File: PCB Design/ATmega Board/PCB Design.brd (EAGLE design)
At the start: 96.3 x 64.3 mm, 33 parts

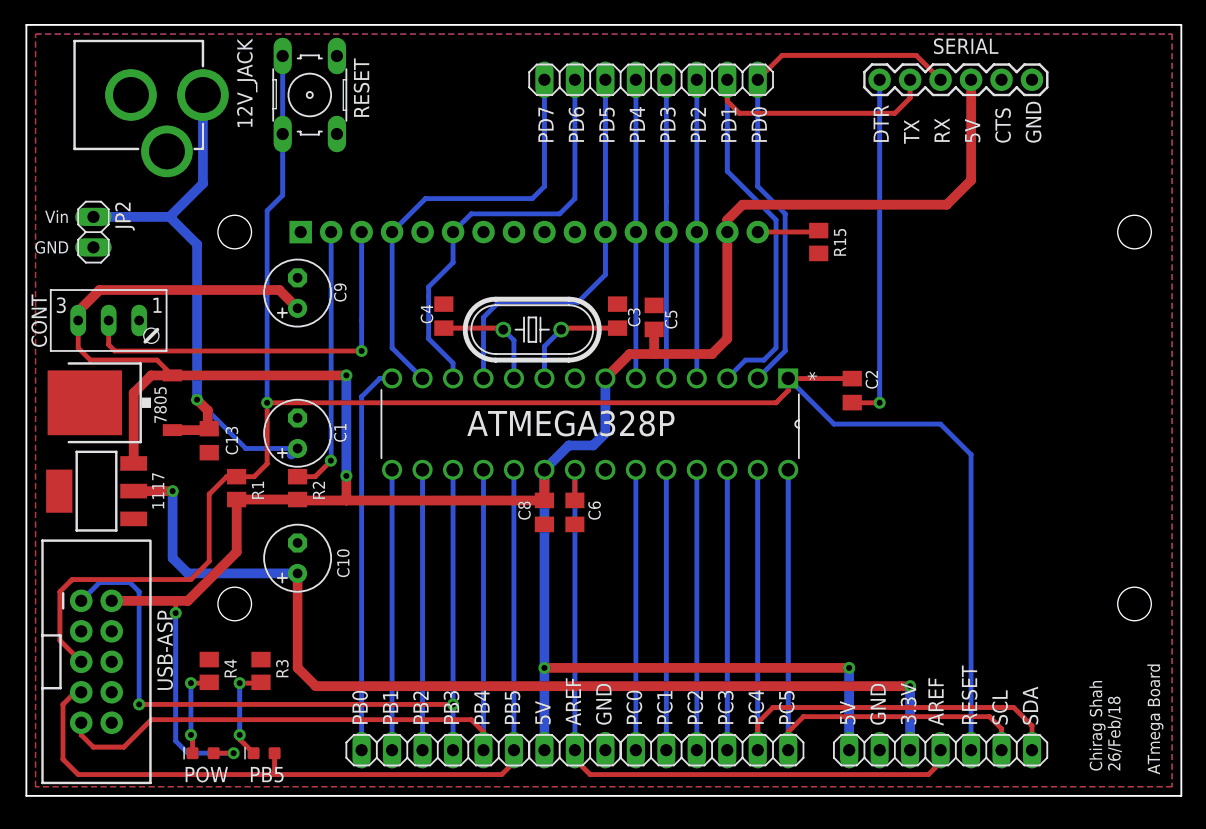
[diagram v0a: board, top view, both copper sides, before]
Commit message: Before renumbering parts
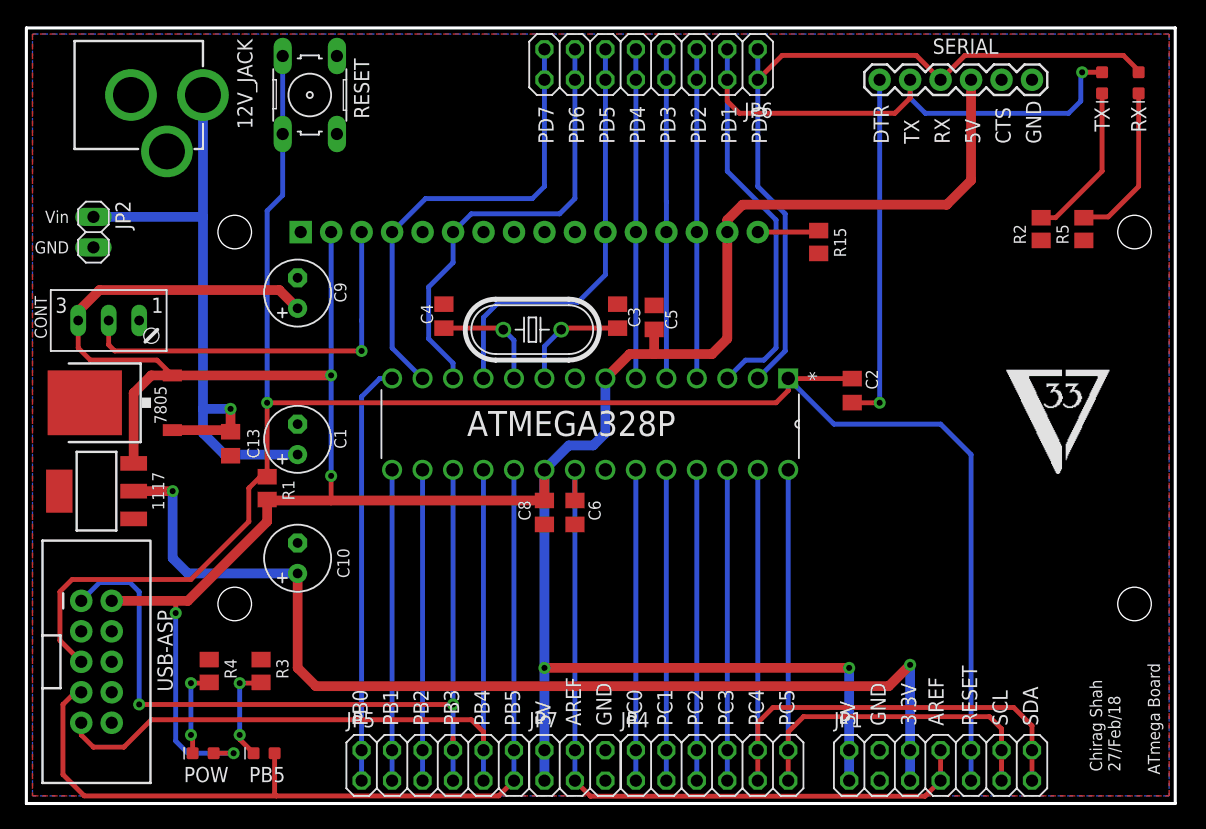
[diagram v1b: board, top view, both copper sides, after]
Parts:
- removed JP3: (no value), pinhead:1X07
- removed PORT_B, PORT_C: (no value), pinhead:1X06
- removed PORT_D: (no value), pinhead:1X08
- added JP4, JP5: (no value), pinhead:2X06
- added JP6: (no value), pinhead:2X08
- added JP7: (no value), pinhead:2X03
- added R5: 330, resistor:M0805
- added RX, TX: BLUE, SparkFun-LED:LED-0603
- JP1: device pinhead:1X03 -> pinhead:2X07
- R2: value 220 -> 330
- moved R2 65.6 mm to (91.9, 53.6)
- moved JP1 30.5 mm to (83.6, 8.89)
- moved R1 2.54 mm to (27.4, 32.0)
- moved C13 1.80 mm to (24.4, 35.7)
- moved C1 0.51 mm to (30.0, 36.1)
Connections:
- new net N$3: R5.2, RX.C
- net +5V: now also JP1.2, JP7.1, JP7.2, LCD.2; no longer JP3.1, R2.1
- net 3.3V: now also JP1.5, JP1.6; no longer JP3.3
- net AREF: now also JP1.7, JP1.8, JP7.3, JP7.4; no longer JP1.2, JP3.4
- net GND: now also JP1.4, JP7.5, JP7.6, R2.1, R5.1; no longer JP3.2
- net N$7: now also TX.C; no longer LCD.2
- net PB0/D8: now also JP5.1, JP5.2; no longer PORT_B.1
- net PB1/D9: now also JP5.3, JP5.4; no longer PORT_B.2
- net PB2/D10: now also JP5.5, JP5.6; no longer PORT_B.3
- net PB3/MOSI/D11: now also JP5.7, JP5.8; no longer PORT_B.4
- net PB4/MISO/D12: now also JP5.10, JP5.9; no longer PORT_B.5
- net PB5/SCK/D13: now also JP5.11, JP5.12; no longer PORT_B.6
- net PC0/A0: now also JP4.1, JP4.2; no longer PORT_C.1
- net PC1/A1: now also JP4.3, JP4.4; no longer PORT_C.2
- net PC2/A2: now also JP4.5, JP4.6; no longer PORT_C.3
- net PC3/A3: now also JP4.7, JP4.8; no longer PORT_C.4
- net PC4/A4/SDA: now also JP1.13, JP1.14, JP4.10, JP4.9; no longer JP3.7, PORT_C.5
- net PC5/A5/SCL: now also JP1.11, JP1.12, JP4.11, JP4.12; no longer JP3.6, PORT_C.6
- net PC6/RESET: now also JP1.10, JP1.9; no longer JP3.5
- net PD0/RX: now also JP6.1, JP6.2, RX.A; no longer PORT_D.1
- net PD1/TX: now also JP6.3, JP6.4, TX.A; no longer PORT_D.2
- net PD2/LCD_D7: now also JP6.5, JP6.6; no longer PORT_D.3
- net PD3/LCD_D6: now also JP6.7, JP6.8; no longer PORT_D.4
- net PD4/LCD_D5: now also JP6.10, JP6.9; no longer PORT_D.5
- net PD5/LCD_D4: now also JP6.11, JP6.12; no longer PORT_D.6
- net PD6/LCD_E: now also JP6.13, JP6.14; no longer PORT_D.7
- net PD7/LCD_RS: now also JP6.15, JP6.16; no longer PORT_D.8
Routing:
- net PD1/TX: track 48.6 -> 72.0 mm, vias 0 -> 1
- net PD0/RX: track 43.7 -> 64.3 mm
- net +5V: track 249.6 -> 263.9 mm
- net N$3: track 0.00 -> 13.4 mm
- net N$7: track 22.4 -> 13.2 mm, vias 1 -> 0
- net PC5/A5/SCL: track 45.4 -> 50.5 mm
- net PC4/A4/SDA: track 51.7 -> 56.8 mm
- net 3.3V: track 84.7 -> 89.7 mm
- net PB5/SCK/D13: track 71.3 -> 76.2 mm
- net +12V: track 50.7 -> 55.1 mm
- net AREF: track 59.1 -> 62.6 mm
- net PB3/MOSI/D11: track 65.7 -> 68.3 mm
- net PD5/LCD_D4: track 33.0 -> 35.5 mm
- net PC3/A3: track 23.4 -> 25.9 mm
- net PC2/A2: track 23.4 -> 25.9 mm
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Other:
- board size 96.3 x 64.3 mm -> 95.8 x 64.6 mm
- board text added: "Chirag Shah 27/Feb/18"
- board text removed: "Chirag Shah 26/Feb/18"
